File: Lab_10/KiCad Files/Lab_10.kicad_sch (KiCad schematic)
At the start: 47 parts

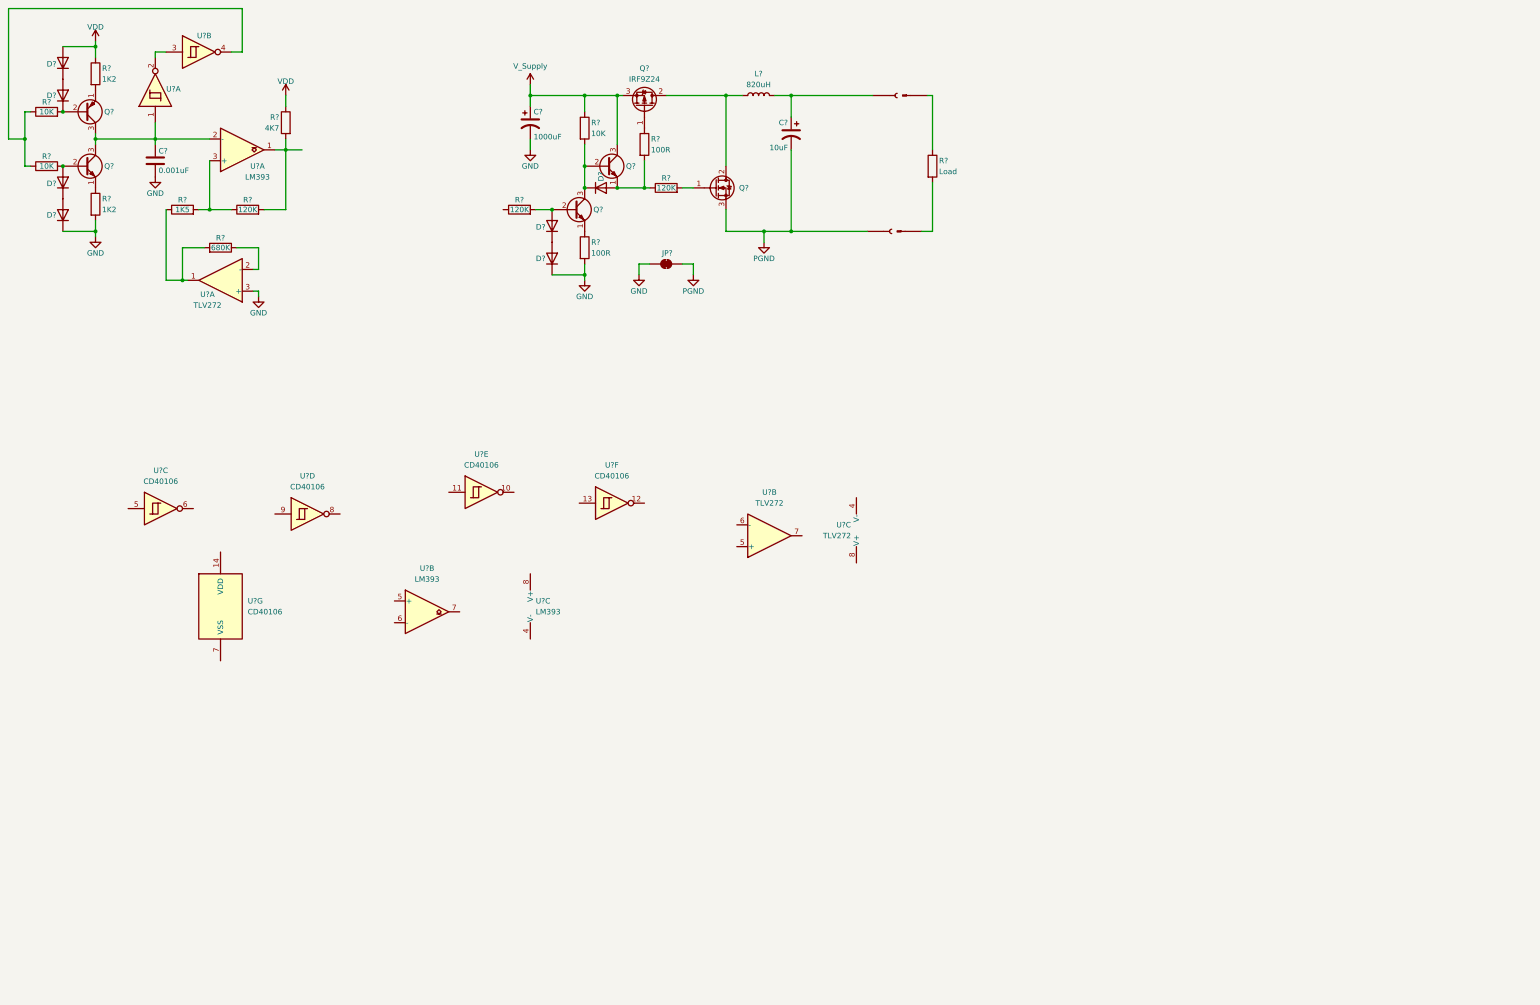
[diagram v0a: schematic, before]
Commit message: Finish Lab 10 Schematic
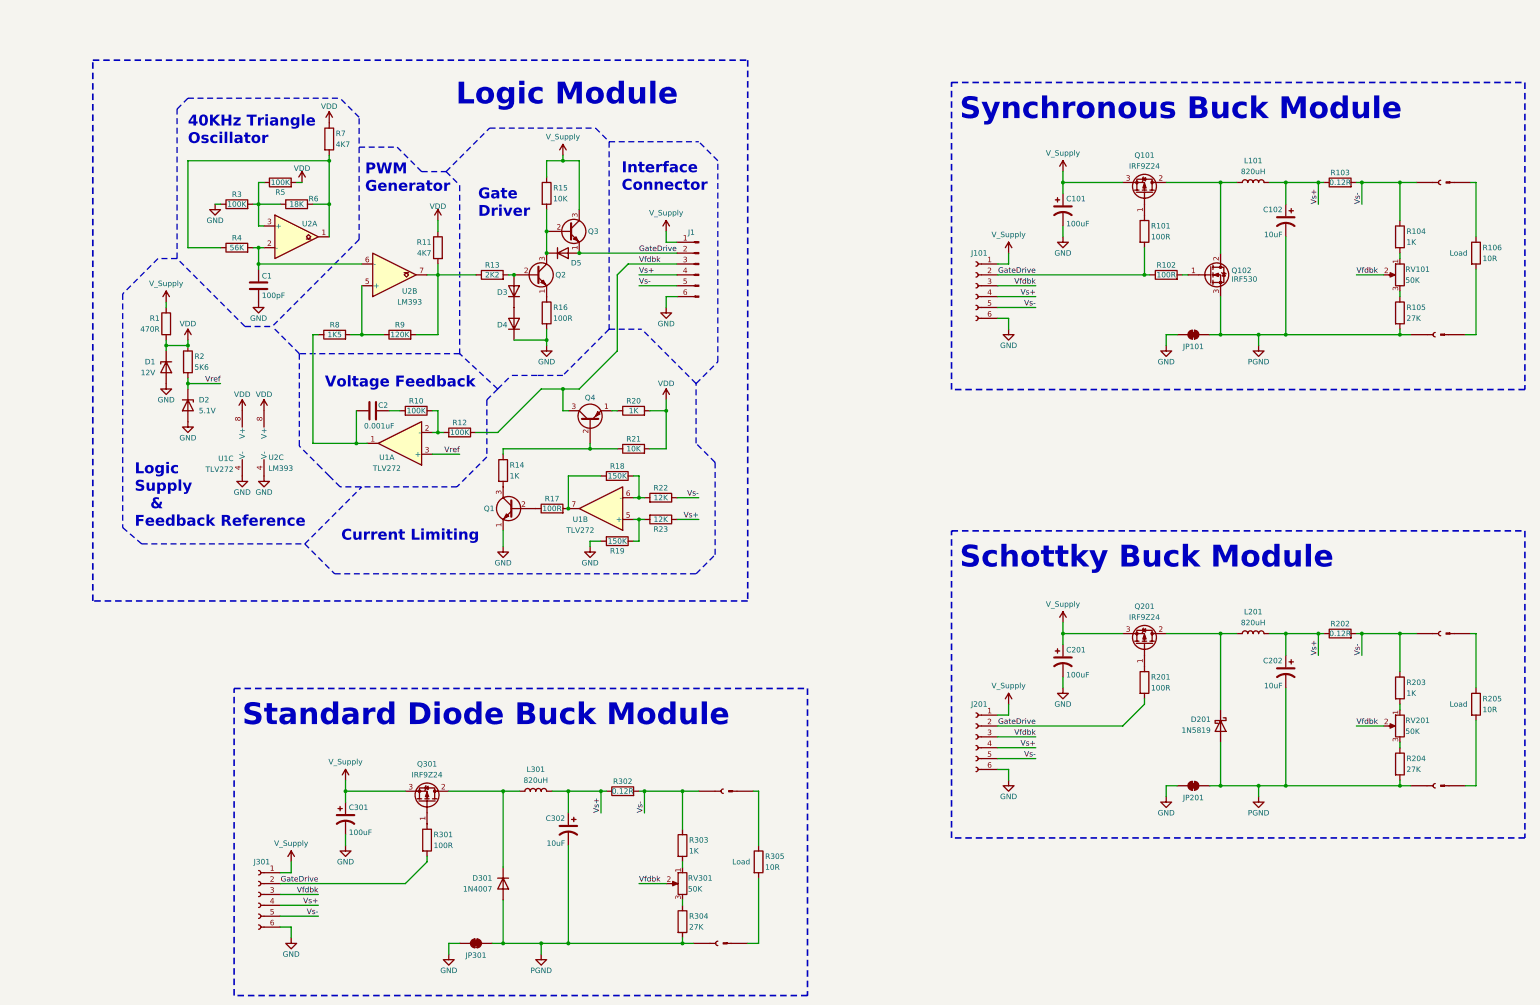
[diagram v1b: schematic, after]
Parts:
- removed D? (x6): D, symbol Device:D
- removed Q? (x3): Q_NPN_EBC, symbol Device:Q_NPN_EBC
- removed Q?: Q_PNP_EBC, symbol Device:Q_PNP_EBC
- removed R? (x2): 10K, symbol Device:R
- removed R? (x2): 1K2, symbol Device:R
- removed U? (x7): CD40106, symbol LarryLab:CD40106
- added C2: 0.001uF, symbol Device:C
- added C201, C301: 100uF, symbol Device:C_Polarized_US
- added C202, C302: 10uF, symbol Device:C_Polarized_US
- added D1: 12V, symbol Device:D_Zener
- added D2: 5.1V, symbol Device:D_Zener
- added D201: 1N5819, symbol Device:D_Schottky
- added D301: 1N4007, symbol Device:D
- added D4, D5: D, symbol Device:D
- added J1: Conn_01x06_Pin, symbol Connector:Conn_01x06_Pin
- added J101, J201, J301: Conn_01x06_Socket, symbol Connector:Conn_01x06_Socket
- added J202, J203, J302, J303: Output_Terminal, symbol LarryLab:Output_Terminal
- added JP201, JP301: SolderJumper_2_Bridged, symbol Jumper:SolderJumper_2_Bridged
- added L201, L301: 820uH, symbol Device:L
- added Q1, Q2, Q3: Q_NPN_EBC, symbol Device:Q_NPN_EBC
- added Q201, Q301: IRF9Z24, symbol Device:Q_PMOS_GDS
- added Q4: Q_PNP_EBC, symbol Device:Q_PNP_EBC
- added R1: 470R, Resistor_THT:R_Axial_DIN0207_L6.3mm_D2.5mm_P7.62mm_Horizontal, symbol Device:R
- added R103, R202, R302: 0.12R, Resistor_THT:R_Axial_DIN0207_L6.3mm_D2.5mm_P7.62mm_Horizontal, symbol Device:R
- added R104, R14, R20, R203, R303: 1K, Resistor_THT:R_Axial_DIN0207_L6.3mm_D2.5mm_P7.62mm_Horizontal, symbol Device:R
- added R105, R204, R304: 27K, Resistor_THT:R_Axial_DIN0207_L6.3mm_D2.5mm_P7.62mm_Horizontal, symbol Device:R
- added R12, R3, R5: 100K, Resistor_THT:R_Axial_DIN0207_L6.3mm_D2.5mm_P7.62mm_Horizontal, symbol Device:R
- added R17, R201, R301: 100R, Resistor_THT:R_Axial_DIN0207_L6.3mm_D2.5mm_P7.62mm_Horizontal, symbol Device:R
- added R18, R19: 150K, Resistor_THT:R_Axial_DIN0207_L6.3mm_D2.5mm_P7.62mm_Horizontal, symbol Device:R
- added R2: 5K6, Resistor_THT:R_Axial_DIN0207_L6.3mm_D2.5mm_P7.62mm_Horizontal, symbol Device:R
- added R205, R305: 10R, Resistor_THT:R_Axial_DIN0207_L6.3mm_D2.5mm_P7.62mm_Horizontal, symbol Device:R
- added R21: 10K, Resistor_THT:R_Axial_DIN0207_L6.3mm_D2.5mm_P7.62mm_Horizontal, symbol Device:R
- added R22, R23: 12K, Resistor_THT:R_Axial_DIN0207_L6.3mm_D2.5mm_P7.62mm_Horizontal, symbol Device:R
- added R4: 56K, Resistor_THT:R_Axial_DIN0207_L6.3mm_D2.5mm_P7.62mm_Horizontal, symbol Device:R
- added R6: 18K, Resistor_THT:R_Axial_DIN0207_L6.3mm_D2.5mm_P7.62mm_Horizontal, symbol Device:R
- added R7: 4K7, Resistor_THT:R_Axial_DIN0207_L6.3mm_D2.5mm_P7.62mm_Horizontal, symbol Device:R
- added RV101, RV201, RV301: 50K, symbol Device:R_Potentiometer
- C1: renamed from C?; value 0.001uF -> 100pF
- C101: renamed from C?; value 1000uF -> 100uF
- Q102: renamed from Q?; value Q_NMOS_GDS -> IRF530
- R10: renamed from R?; value 680K -> 100K; footprint (none) -> Resistor_THT:R_Axial_DIN0207_L6.3mm_D2.5mm_P7.62mm_Horizontal
- R101, R11, R15, R16, R8, R9: renamed from R?; footprint (none) -> Resistor_THT:R_Axial_DIN0207_L6.3mm_D2.5mm_P7.62mm_Horizontal
- R102: renamed from R?; value 120K -> 100R; footprint (none) -> Resistor_THT:R_Axial_DIN0207_L6.3mm_D2.5mm_P7.62mm_Horizontal
- R106: renamed from R?; value Load -> 10R; footprint (none) -> Resistor_THT:R_Axial_DIN0207_L6.3mm_D2.5mm_P7.62mm_Horizontal
- R13: renamed from R?; value 120K -> 2K2; footprint (none) -> Resistor_THT:R_Axial_DIN0207_L6.3mm_D2.5mm_P7.62mm_Horizontal
- gave numbers to parts that had none: 9
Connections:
- net GND: now also U1.4 (V-), U2.4 (V-), C201.2, C301.2, D1.2 (A), D2.2 (A), D4.1 (K), J1.6 (Pin_6), J101.6 (Pin_6), J201.6 (Pin_6), J301.6 (Pin_6), JP201.1 (A), JP301.1 (A), Q1.1 (E), R19.2, R3.1; no longer U1.3 (+)
- net PGND: now also C202.2, C302.2, D201.2 (A), D301.2 (A), J202.1 (In), J302.1 (In), JP201.2 (B), JP301.2 (B), R105.2, R204.2, R304.2
- net VDD: now also U1.8 (V+), U2.8 (V+), D1.1 (K), R1.2, R2.1, R20.2, R21.2, R5.2, R7.1
- net V_Supply: now also C201.1, C301.1, J1.1 (Pin_1), J101.1 (Pin_1), J201.1 (Pin_1), J301.1 (Pin_1), Q201.3 (S), Q3.3 (C), Q301.3 (S), R1.1
- net at R15.2: now also D5.1 (K), Q2.3 (C), Q3.2 (B)
- net at R8.1, U1.1: now also C2.1; no longer R10.2
- net at R8.2, R9.1: now also U2.5 (+); no longer U2.3 (+)
- net at D3.1 (K): now also D4.2 (A)
- net at R10.1, U1.2 (-): now also R12.2
- net at U1.5 (+): now also R19.1, R23.2
- net at U1.6 (-): now also R18.1, R22.2
- net at U1.7: now also R17.2, R18.2
- net at R11.2, R9.2: now also R13.1, U2.7; no longer U2.1
- net at C1.1: now also U2.2 (-), U2.6 (-), R4.2; no longer U2.2 (-)
- net at R16.1: now also Q2.1 (E)
- net GateDrive: now reaches R101.2, R102.1
- net GateDrive: now also D5.2 (A), J1.2 (Pin_2), J101.2 (Pin_2), J201.2 (Pin_2), J301.2 (Pin_2), Q3.1 (E), R201.2, R301.2
- net at D3.2 (A), R13.2: now also Q2.2 (B)
- net Vs+: now reaches C102.1, L101.2
- net Vs+: now also C202.1, C302.1, J1.4 (Pin_4), J101.4 (Pin_4), J201.4 (Pin_4), J301.4 (Pin_4), L201.2, L301.2, R103.1, R202.1, R23.1, R302.1; no longer J103.1 (In)
- new net: D201.1 (K), L201.1, Q201.2 (D)
- new net: Q1.2 (B), R17.1
- new net: Q1.3 (C), R14.2
- new net: J302.2 (Out), R305.2
- new net: R303.2, RV301.1
- new net: R304.1, RV301.3
- new net: D301.1 (K), L301.1, Q301.2 (D)
- new net: R4.1, R6.2, R7.2, U2.1
- new net: R3.2, R5.1, R6.1, U2.3 (+)
- new net: Q201.1 (G), R201.1
- new net: Q301.1 (G), R301.1
- new net: C2.2, R10.2
- new net: J203.2 (Out), R205.1
- new net: J303.2 (Out), R305.1
- new net: J202.2 (Out), R205.2
- new net: Q4.1 (E), R20.1
- new net: R204.1, RV201.3
- new net: Q4.2 (B), R14.1, R21.1
- new net: R104.2, RV101.1
- new net: R105.1, RV101.3
- new net: R203.2, RV201.1
- new net Vfdbk: J1.3 (Pin_3), J101.3 (Pin_3), J201.3 (Pin_3), J301.3 (Pin_3), Q4.3 (C), R12.1, RV101.2, RV201.2, RV301.2
- new net Vref: D2.1 (K), R2.2, U1.3 (+)
- new net Vs-: J1.5 (Pin_5), J101.5 (Pin_5), J103.1 (In), J201.5 (Pin_5), J203.1 (In), J301.5 (Pin_5), J303.1 (In), R103.2, R104.1, R202.2, R203.1, R22.1, R302.2, R303.1
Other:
- note added: "40KHz Triangle Oscillator"
- note added: "Current Limiting"
- note added: "Gate Driver"
- note added: "Interface Connector"
- note added: "Logic Module"
- note added: "Logic Supply & Feedback Reference"
- note added: "PWM Generator"
- note added: "Schottky Buck Module"
- note added: "Standard Diode Buck Module"
- note added: "Synchronous Buck Module"
- note added: "Voltage Feedback"
- company: (none) -> ZAM Industries, LLC
- title: (none) -> Switching DC-DC Buck Converters
- moved on the sheet: C1, C101, C102, D3, JP101, L101, Q101, Q102, R10, R101, R102, R106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

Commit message: Complete Lab 10
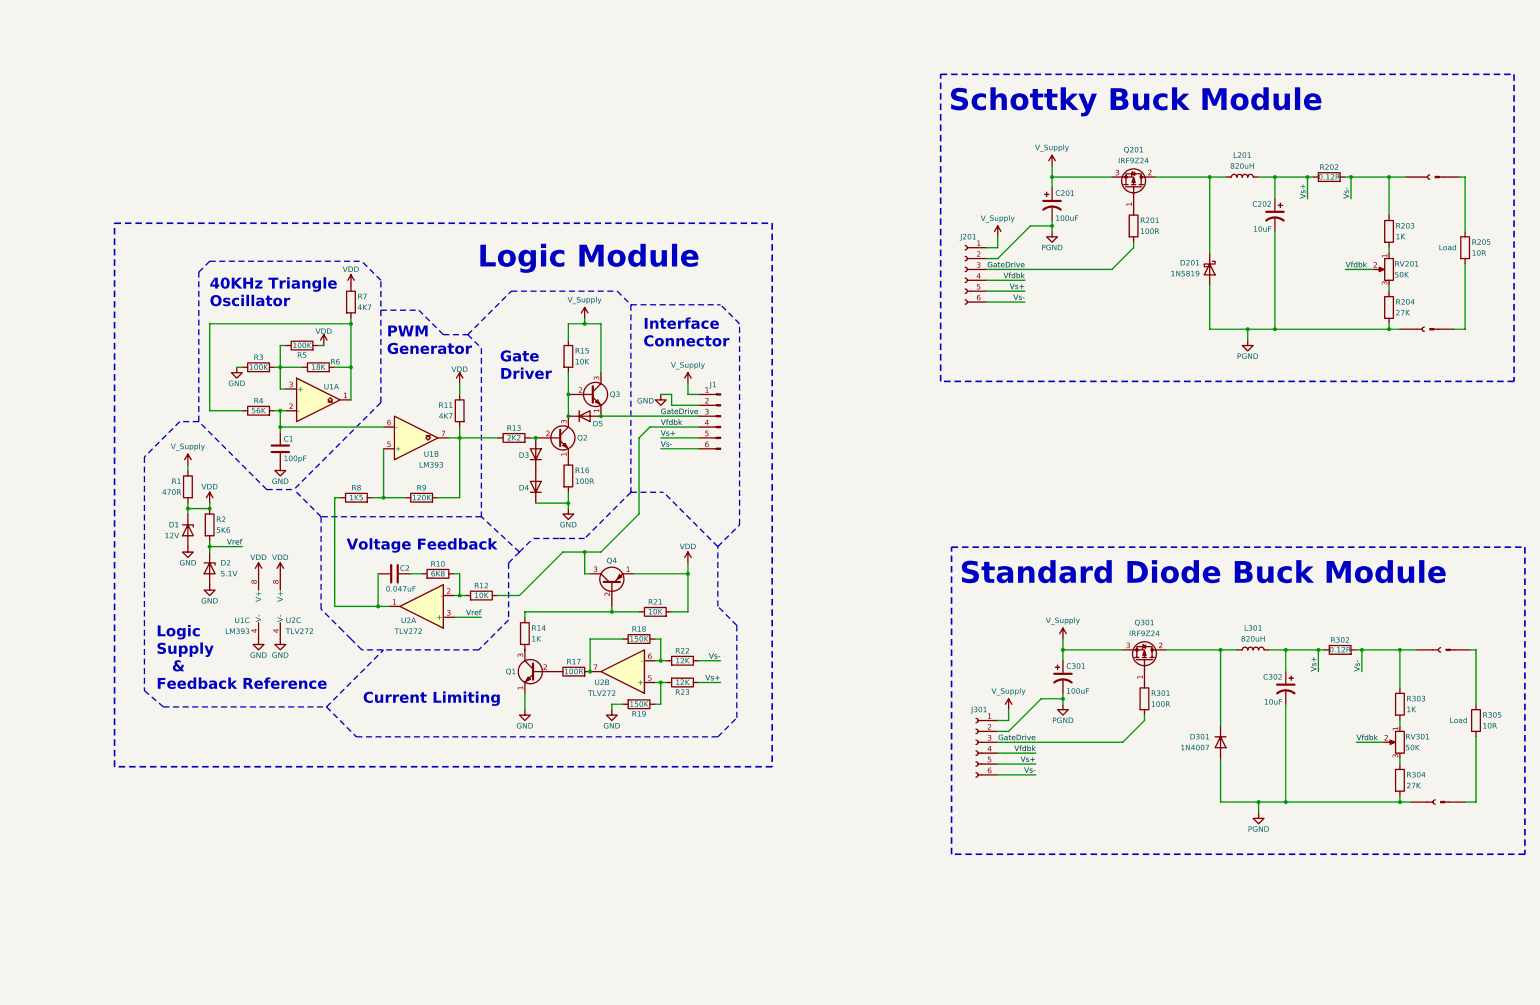
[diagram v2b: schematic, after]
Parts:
- removed C101: 100uF, symbol Device:C_Polarized_US
- removed C102: 10uF, symbol Device:C_Polarized_US
- removed J101: Conn_01x06_Socket, symbol Connector:Conn_01x06_Socket
- removed J102, J103: Output_Terminal, symbol LarryLab:Output_Terminal
- removed JP101, JP201, JP301: SolderJumper_2_Bridged, symbol Jumper:SolderJumper_2_Bridged
- removed L101: 820uH, symbol Device:L
- removed Q101: IRF9Z24, symbol Device:Q_PMOS_GDS
- removed Q102: IRF530, symbol Device:Q_NMOS_GDS
- removed R101, R102: 100R, Resistor_THT:R_Axial_DIN0207_L6.3mm_D2.5mm_P7.62mm_Horizontal, symbol Device:R
- removed R103: 0.12R, Resistor_THT:R_Axial_DIN0207_L6.3mm_D2.5mm_P7.62mm_Horizontal, symbol Device:R
- removed R104, R20: 1K, Resistor_THT:R_Axial_DIN0207_L6.3mm_D2.5mm_P7.62mm_Horizontal, symbol Device:R
- removed R105: 27K, Resistor_THT:R_Axial_DIN0207_L6.3mm_D2.5mm_P7.62mm_Horizontal, symbol Device:R
- removed R106: 10R, Resistor_THT:R_Axial_DIN0207_L6.3mm_D2.5mm_P7.62mm_Horizontal, symbol Device:R
- removed RV101: 50K, symbol Device:R_Potentiometer
- C2: value 0.001uF -> 0.047uF
- J201, J301: footprint (none) -> Connector_PinHeader_2.54mm:PinHeader_1x06_P2.54mm_Vertical
- R10: value 100K -> 6K8
- R12: value 100K -> 10K
- renumbered U2 to U1, U1 to U2
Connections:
- net GND: now also J1.2 (Pin_2); no longer C201.2, C301.2, J1.6 (Pin_6), J201.6 (Pin_6), J301.6 (Pin_6)
- net GateDrive: now also J1.3 (Pin_3), J201.3 (Pin_3), J301.3 (Pin_3); no longer J1.2 (Pin_2), J201.2 (Pin_2), J301.2 (Pin_2)
- net PGND: now also C201.2, C301.2, J201.2 (Pin_2), J301.2 (Pin_2)
- net VDD: now also Q4.1 (E)
- net Vfdbk: now also J1.4 (Pin_4), J201.4 (Pin_4), J301.4 (Pin_4); no longer J1.3 (Pin_3), J201.3 (Pin_3), J301.3 (Pin_3)
- net Vs+: now also J1.5 (Pin_5), J201.5 (Pin_5), J301.5 (Pin_5); no longer J1.4 (Pin_4), J201.4 (Pin_4), J301.4 (Pin_4)
- net Vs-: now also J1.6 (Pin_6), J201.6 (Pin_6), J301.6 (Pin_6); no longer J1.5 (Pin_5), J201.5 (Pin_5), J301.5 (Pin_5)
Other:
- note removed: "Synchronous Buck Module"
- moved on the sheet: C1, C2, C201, C202, C301, C302, D1, D2, D201, D3, D301, J1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
